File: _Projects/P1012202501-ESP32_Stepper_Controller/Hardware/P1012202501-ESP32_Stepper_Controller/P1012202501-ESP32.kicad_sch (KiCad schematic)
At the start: 14 parts, among them IC3 ESP32-WROOM-32UE-N16, J4 KH68001-406HLF

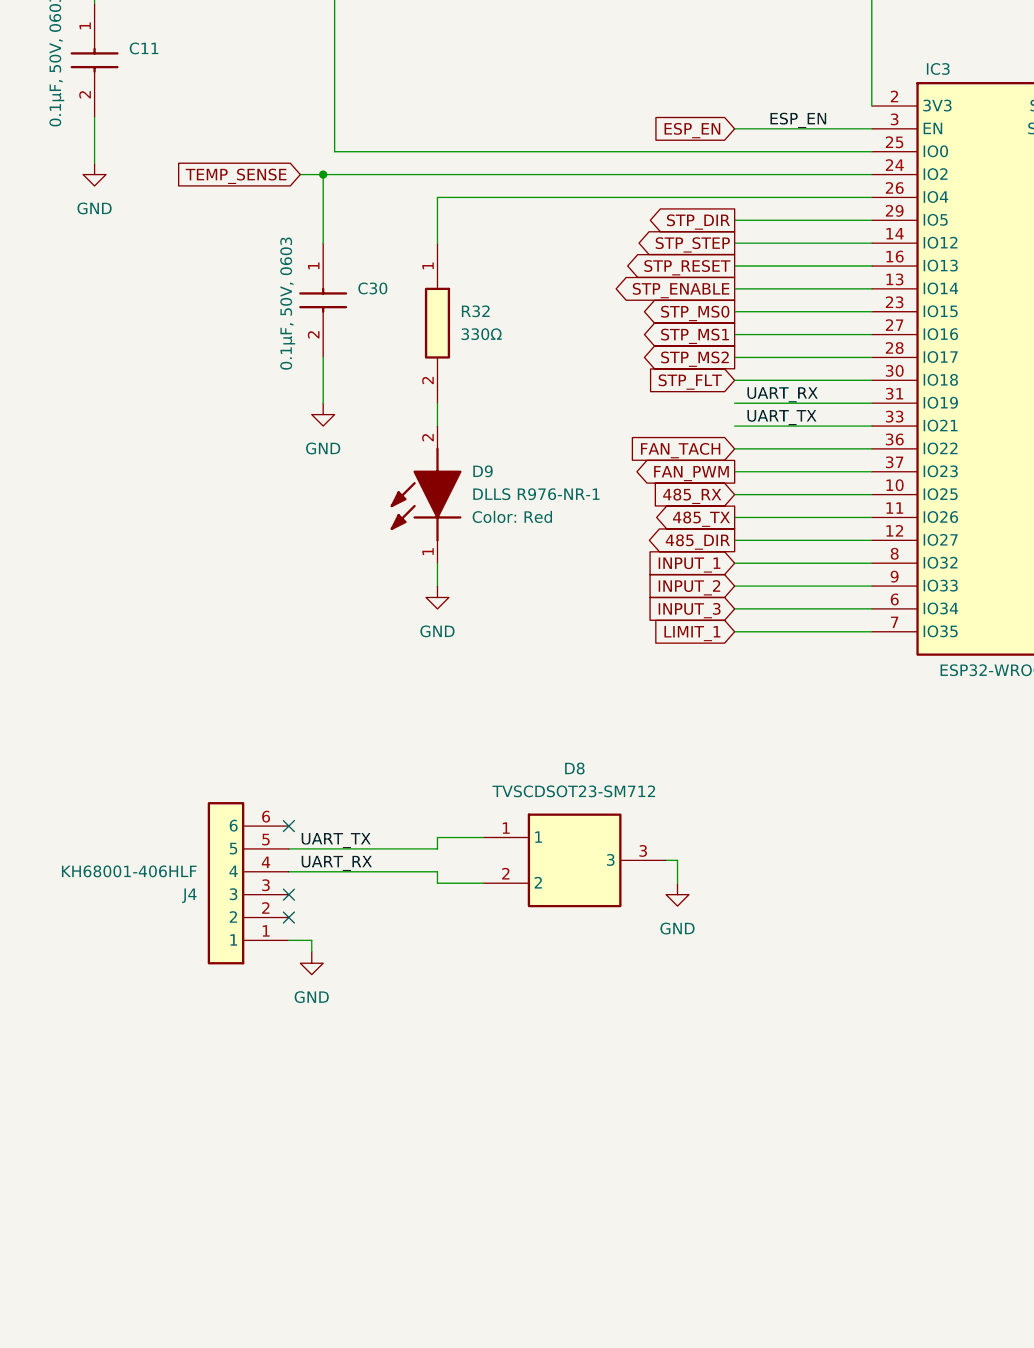
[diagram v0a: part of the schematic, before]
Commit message: Adding new items from recent streams.
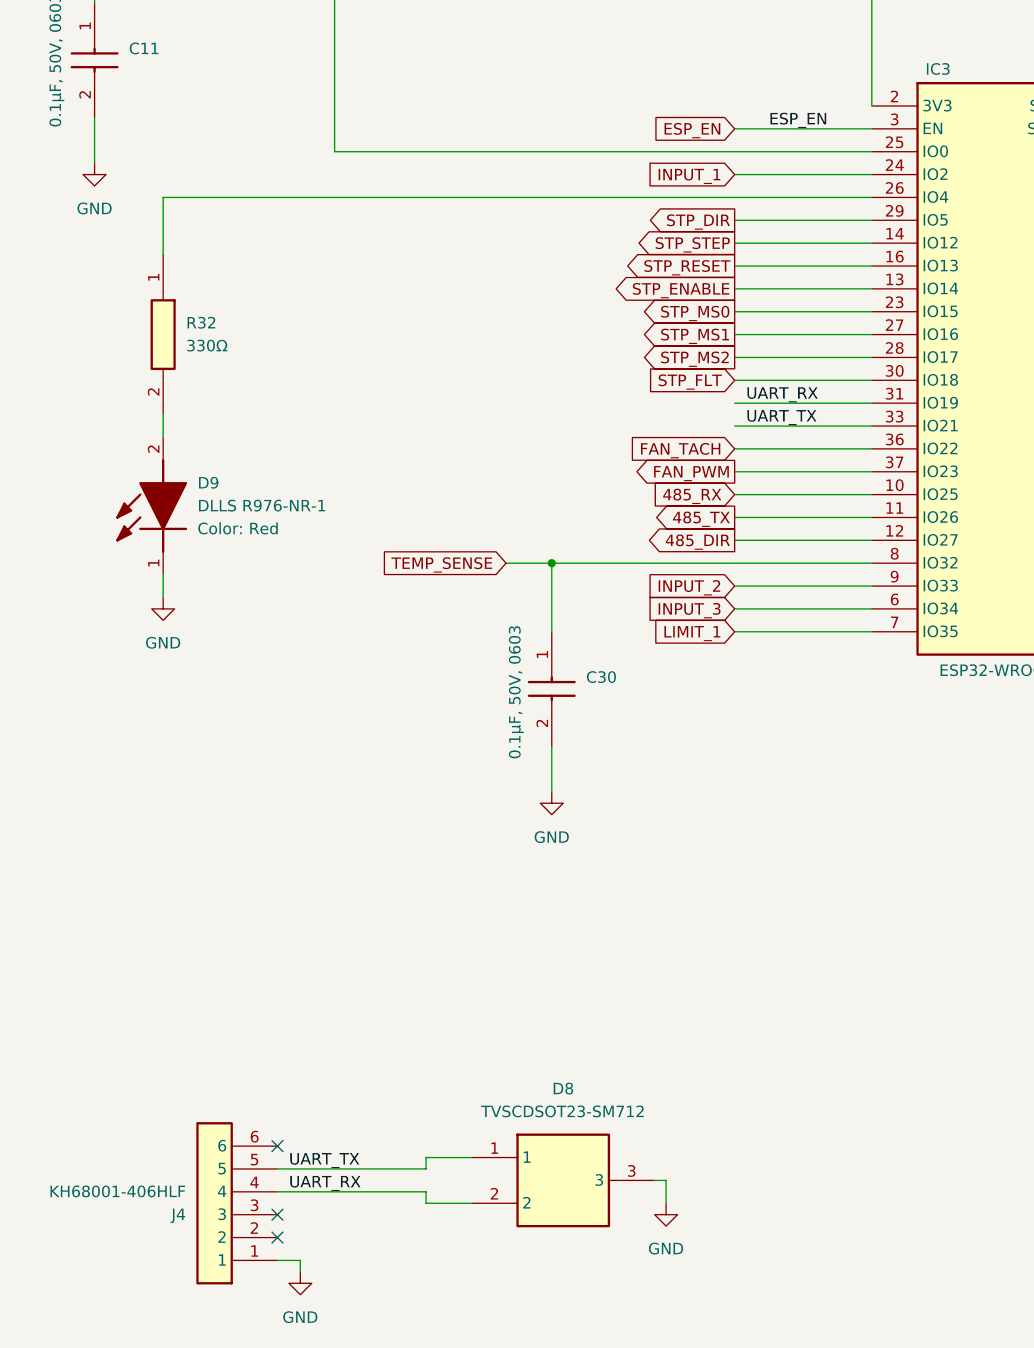
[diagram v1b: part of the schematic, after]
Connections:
- net INPUT_1: now also IC3.24 (IO2); no longer IC3.8 (IO32)
- net TEMP_SENSE: now also IC3.8 (IO32); no longer IC3.24 (IO2)
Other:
- moved on the sheet: C30, D8, D9, J4, R32
